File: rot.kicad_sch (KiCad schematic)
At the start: 35 parts, among them J4 PinSocket_2x6_P2.54mm_Drill1.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, J8 Plug_Molex_SlimStack_2x25_529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, U2 W25Q32JW_SOIC-8, U3 W25Q32JW_SOIC-8, U4 W25Q32JW_SOIC-8, U5 W25Q32JW_SOIC-8

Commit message: version 1.0 complete
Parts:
- R21, R22, R23, R24: MPN CR0402-FX-4701GLF -> RC0402FR-7D4K7L; Manufacturer Bourns -> YAGEO
- R29, R30, R31, R32, R33, R34, R35, R36, R37, R38, R39, R40, R41, R42, R43, R44: MPN CR0402-FX-1002GLF -> CR0402AFX-1002GAS

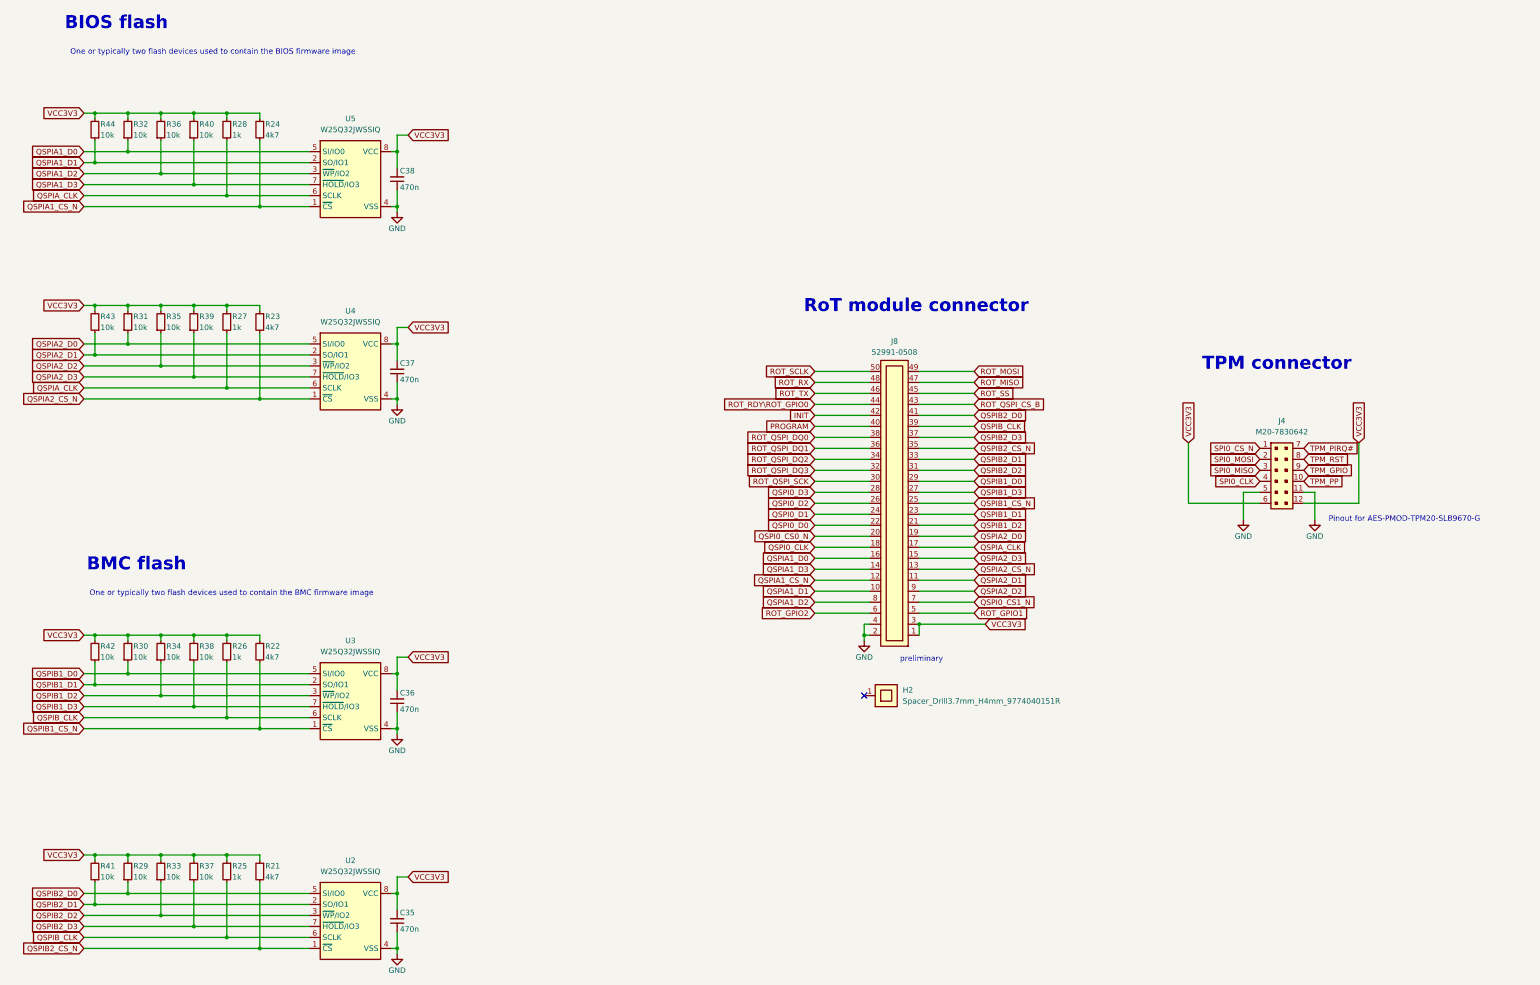
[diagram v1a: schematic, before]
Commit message: "In the process of upgrading the ddr memory"
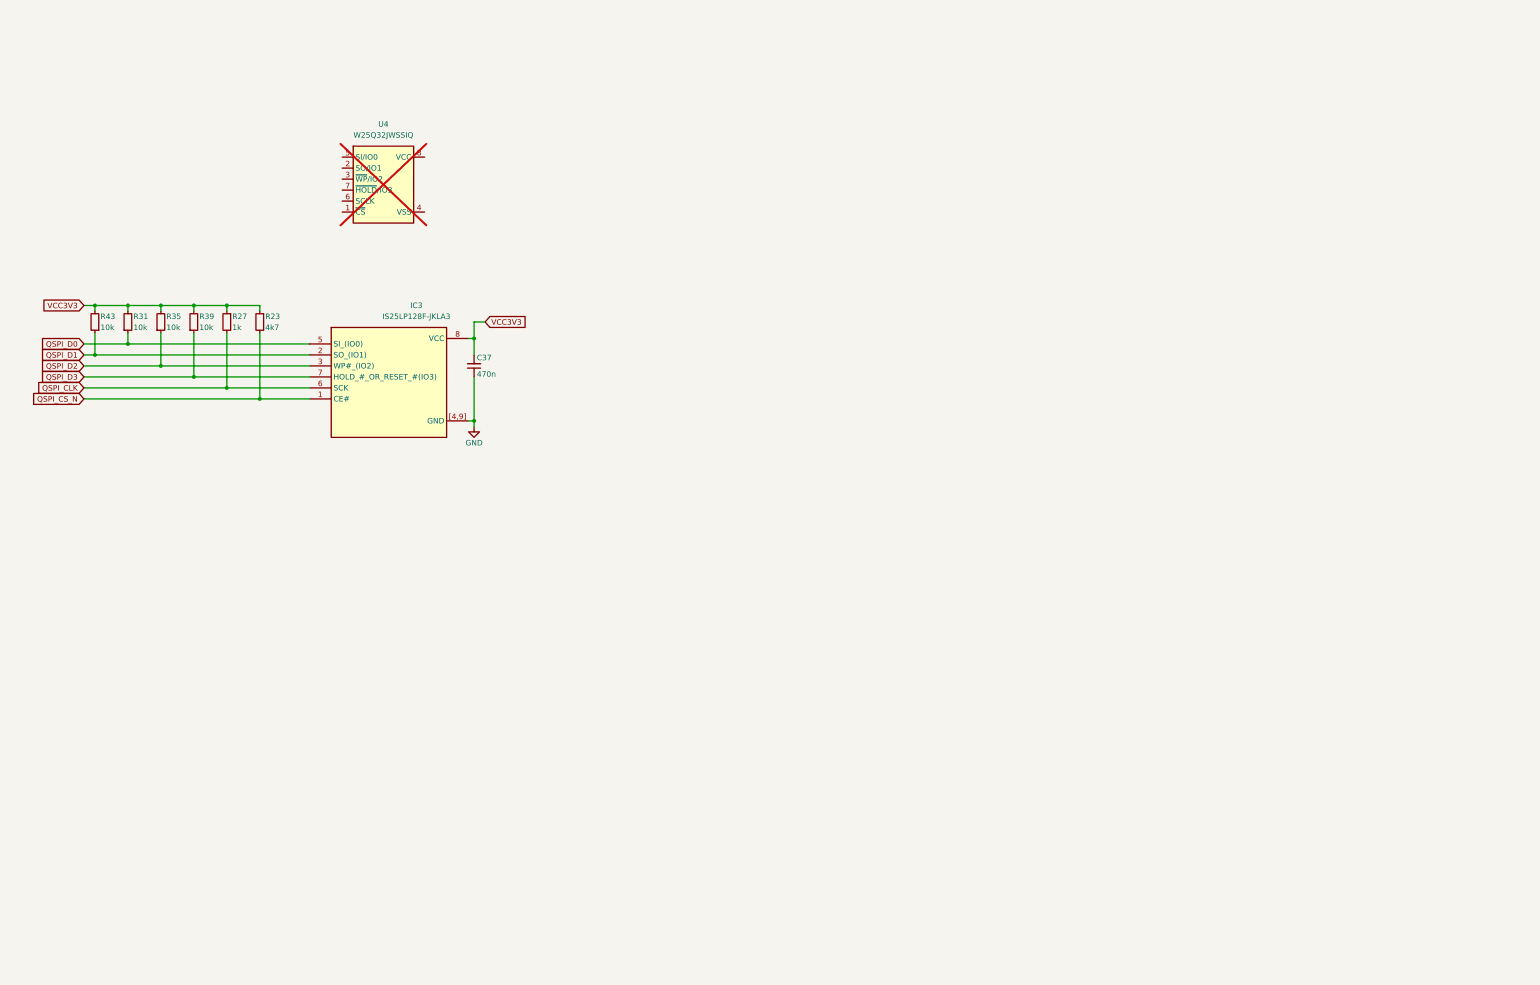
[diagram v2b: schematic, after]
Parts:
- removed C35, C36, C38: C_470n_0402, Capacitor_SMD:C_0402_1005Metric, symbol antmicroCapacitors0402:C_470n_0402
- removed H2: Spacer_Drill3.7mm_H4mm_9774040151R, antmicro-footprints:Spacer_Drill3.7mm_H4mm_9774040151R, symbol antmicroMechanicalParts:Spacer_Drill3.7mm_H4mm_9774040151R
- removed J4: PinSocket_2x6_P2.54mm_Drill1.02mm_PMOD, antmicro-footprints:PinSocket_2x6_P2.54mm_Drill1.02mm_PMOD, symbol antmicroGenericPinSockets:PinSocket_2x6_P2.54mm_Drill1.02mm_PMOD
- removed J8: Plug_Molex_SlimStack_2x25_529910508, antmicro-footprints:Conn_Plug_Molex_SlimStack_2x25_529910508, symbol antmicroB2BConnectors:Plug_Molex_SlimStack_2x25_529910508
- removed R21, R22, R24: R_4k7_0402, antmicro-footprints:R_0402_1005Metric, symbol antmicroResistors0402:R_4k7_0402
- removed R25, R26, R28: R_1k_0402, antmicro-footprints:R_0402_1005Metric, symbol antmicroResistors0402:R_1k_0402
- removed R29, R30, R32, R33, R34, R36, R37, R38, R40, R41, R42, R44: R_10k_0402, antmicro-footprints:R_0402_1005Metric, symbol antmicroResistors0402:R_10k_0402
- removed U2, U3, U5: W25Q32JW_SOIC-8, antmicro-footprints:SOIC-8_5.3x5.3x2mm_P1.27mm, symbol antmicroMemory:W25Q32JW_SOIC-8
- added IC3: IS25LP128F-JKLA3, SON127P600X500X80-9N-D, symbol artix-dc-scm:IS25LP128F-JKLA3
- R23, R27, R31, R35, R39, R43: footprint antmicro-footprints:R_0402_1005Metric -> Resistor_SMD:R_0402_1005Metric
- U4: now not fitted; now left out of the parts list
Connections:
- net GND: now also IC3.[4,9] (GND); no longer U4.4 (VSS)
- net VCC3V3: now also IC3.8 (VCC); no longer U4.8 (VCC)
- net QSPIA2_CS_N: no longer names the net of U4.1 (~{CS})
- net QSPIA2_CS_N: no longer R23.2
- net QSPIA2_D0: no longer names the net of U4.5 (SI/IO0)
- net QSPIA2_D0: no longer R31.1
- net QSPIA2_D1: no longer names the net of U4.2 (SO/IO1)
- net QSPIA2_D1: no longer R43.1
- net QSPIA2_D2: no longer names the net of U4.3 (~{WP}/IO2)
- net QSPIA2_D2: no longer R35.1
- net QSPIA2_D3: no longer names the net of U4.7 (~{HOLD}/IO3)
- net QSPIA2_D3: no longer R39.1
- net QSPIA_CLK: no longer names the net of U4.6 (SCLK)
- net QSPIA_CLK: no longer R27.2
- new net QSPI_CLK: IC3.6 (SCK), R27.2
- new net QSPI_CS_N: IC3.1 (CE#), R23.2
- new net QSPI_D0: IC3.5 (SI_(IO0)), R31.1
- new net QSPI_D1: IC3.2 (SO_(IO1)), R43.1
- new net QSPI_D2: IC3.3 (WP#_(IO2)), R35.1
- new net QSPI_D3: IC3.7 (HOLD_#_OR_RESET_#(IO3)), R39.1
- no-connect marks 1 -> 0
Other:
- note removed: "BIOS flash"
- note removed: "BMC flash"
- note removed: "One or typically two flash devices used to contain the BIOS firmware image"
- note removed: "One or typically two flash devices used to contain the BMC firmware image"
- note removed: "Pinout for AES-PMOD-TPM20-SLB9670-G"
- note removed: "RoT module connector"
- note removed: "TPM connector"
- note removed: "preliminary"
- moved on the sheet: C37
